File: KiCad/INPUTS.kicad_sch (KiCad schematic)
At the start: 8 parts

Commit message: Actualizació Footprints
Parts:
- R_BTNDOWN1, R_BTNUP1, R_LIMIT1, R_MCLR1: footprint (none) -> Resistor_SMD:R_0805_2012Metric
- SW_UP1, SW_UP2, SW_UP3, SW_UP4: footprint (none) -> Button_Switch_SMD:SW_SPST_TL3342
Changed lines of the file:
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@@
 			)
 		)
-		(property "Footprint" ""
+		(property "Footprint" "Resistor_SMD:R_0805_2012Metric"
 			(at 139.7 74.168 90)
 			(effects
@@
 			)
 		)
-		(property "Footprint" ""
+		(property "Footprint" "Resistor_SMD:R_0805_2012Metric"
 			(at 139.7 95.758 90)
 			(effects
@@
 			)
 		)
-		(property "Footprint" ""
+		(property "Footprint" "Button_Switch_SMD:SW_SPST_TL3342"
 			(at 152.4 67.31 0)
 			(effects
@@
 			)
 		)
-		(property "Footprint" ""
+		(property "Footprint" "Resistor_SMD:R_0805_2012Metric"
 			(at 139.7 117.348 90)
 			(effects
@@
 			)
 		)
-		(property "Footprint" ""
+		(property "Footprint" "Resistor_SMD:R_0805_2012Metric"
 			(at 139.7 51.308 90)
 			(effects
@@
 			)
 		)
-		(property "Footprint" ""
+		(property "Footprint" "Button_Switch_SMD:SW_SPST_TL3342"
 			(at 152.4 88.9 0)
 			(effects
@@
 			)
 		)
-		(property "Footprint" ""
+		(property "Footprint" "Button_Switch_SMD:SW_SPST_TL3342"
 			(at 152.4 110.49 0)
 			(effects
@@
 			)
 		)
-		(property "Footprint" ""
+		(property "Footprint" "Button_Switch_SMD:SW_SPST_TL3342"
 			(at 152.4 44.45 0)
 			(effects

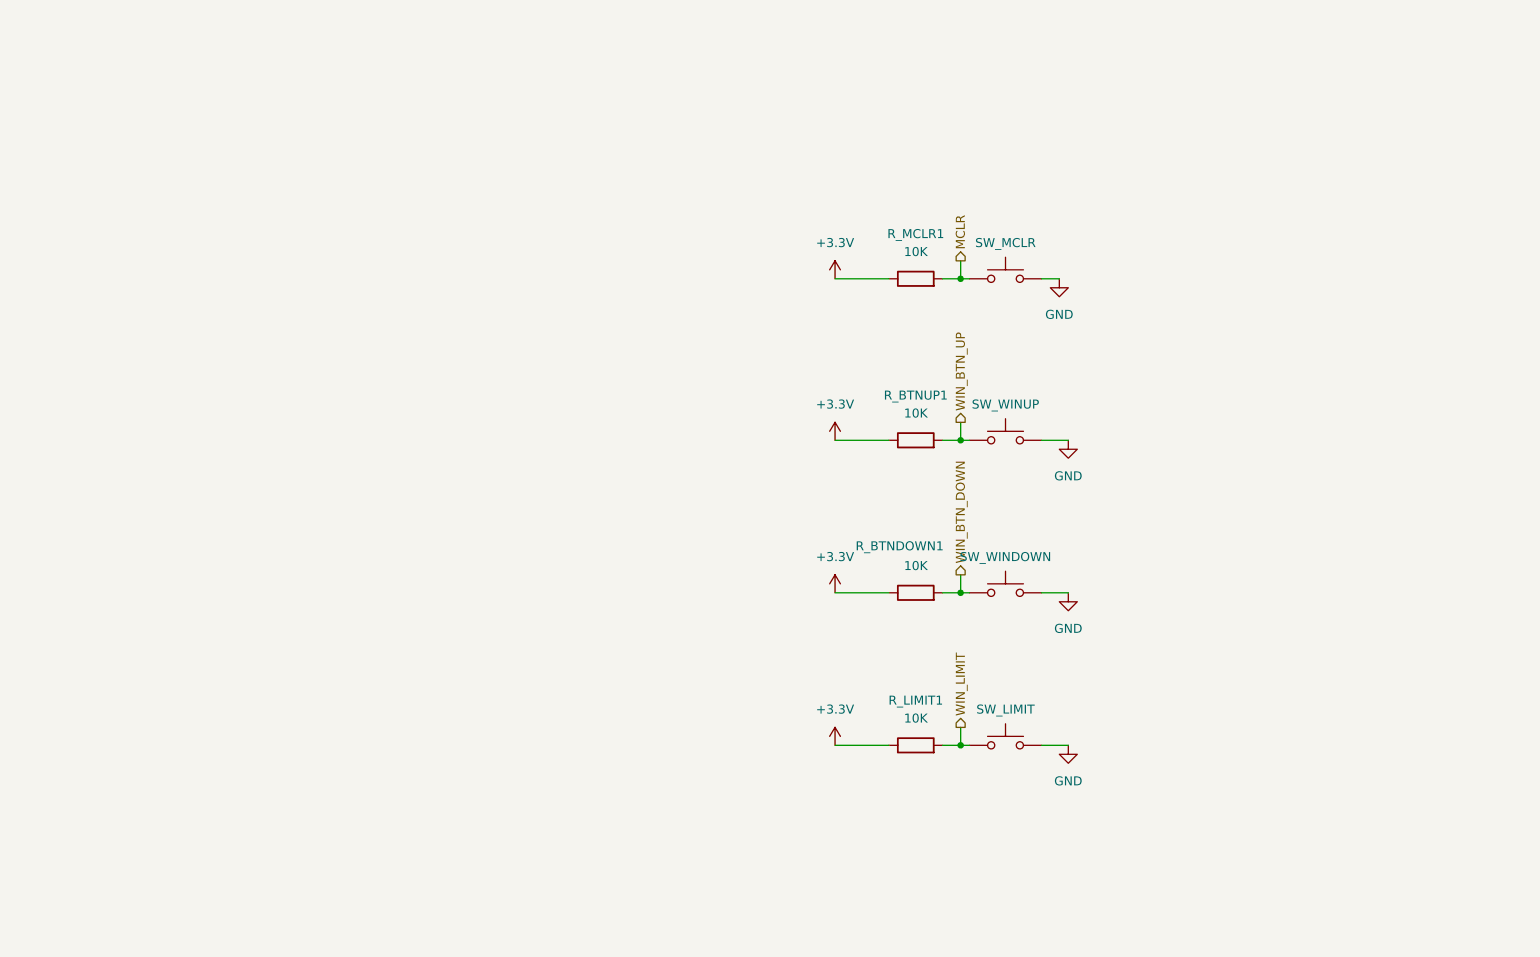
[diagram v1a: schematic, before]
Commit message: Versió final Esquematic
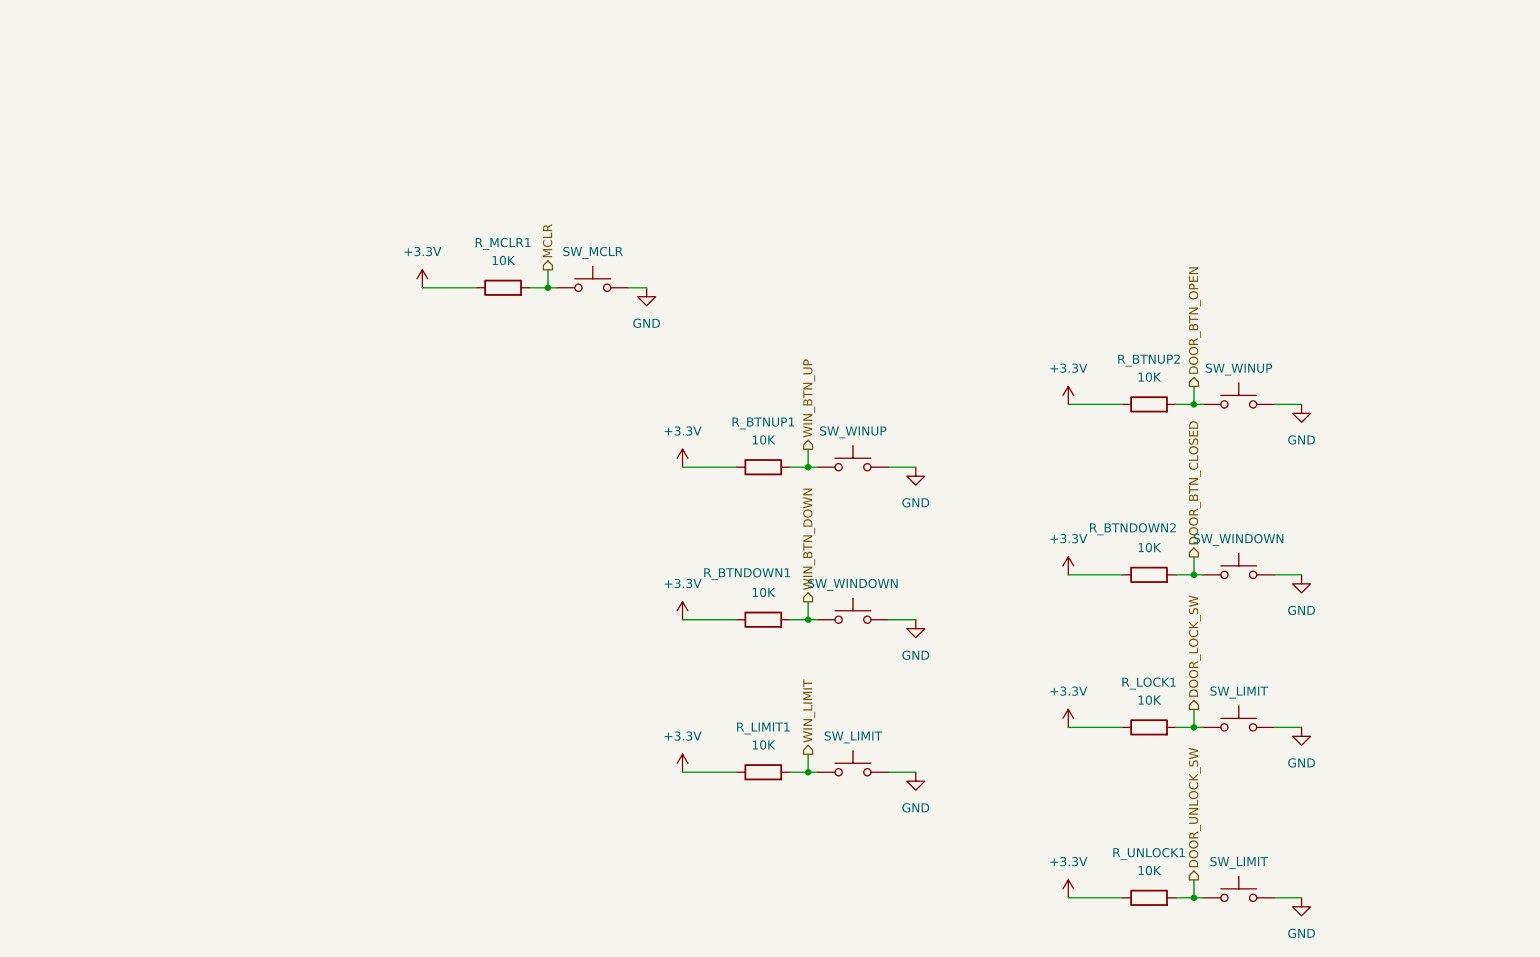
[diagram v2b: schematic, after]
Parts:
- added R_BTNDOWN2, R_BTNUP2, R_LOCK1, R_UNLOCK1: 10K, Resistor_SMD:R_0805_2012Metric, symbol Device:R
- added SW_UP5: SW_WINUP, Button_Switch_SMD:SW_SPST_TL3342, symbol Switch:SW_Push
- added SW_UP6: SW_WINDOWN, Button_Switch_SMD:SW_SPST_TL3342, symbol Switch:SW_Push
- added SW_UP7, SW_UP8: SW_LIMIT, Button_Switch_SMD:SW_SPST_TL3342, symbol Switch:SW_Push
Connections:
- net +3.3V: now also R_BTNDOWN2.1, R_BTNUP2.1, R_LOCK1.1, R_UNLOCK1.1
- net GND: now also SW_UP5.2, SW_UP6.2, SW_UP7.2, SW_UP8.2
- new net DOOR_BTN_CLOSED: R_BTNDOWN2.2, SW_UP6.1
- new net DOOR_BTN_OPEN: R_BTNUP2.2, SW_UP5.1
- new net DOOR_LOCK_SW: R_LOCK1.2, SW_UP7.1
- new net DOOR_UNLOCK_SW: R_UNLOCK1.2, SW_UP8.1
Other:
- moved on the sheet: R_BTNDOWN1, R_BTNUP1, R_LIMIT1, R_MCLR1

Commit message: Versió final de l'esquematic
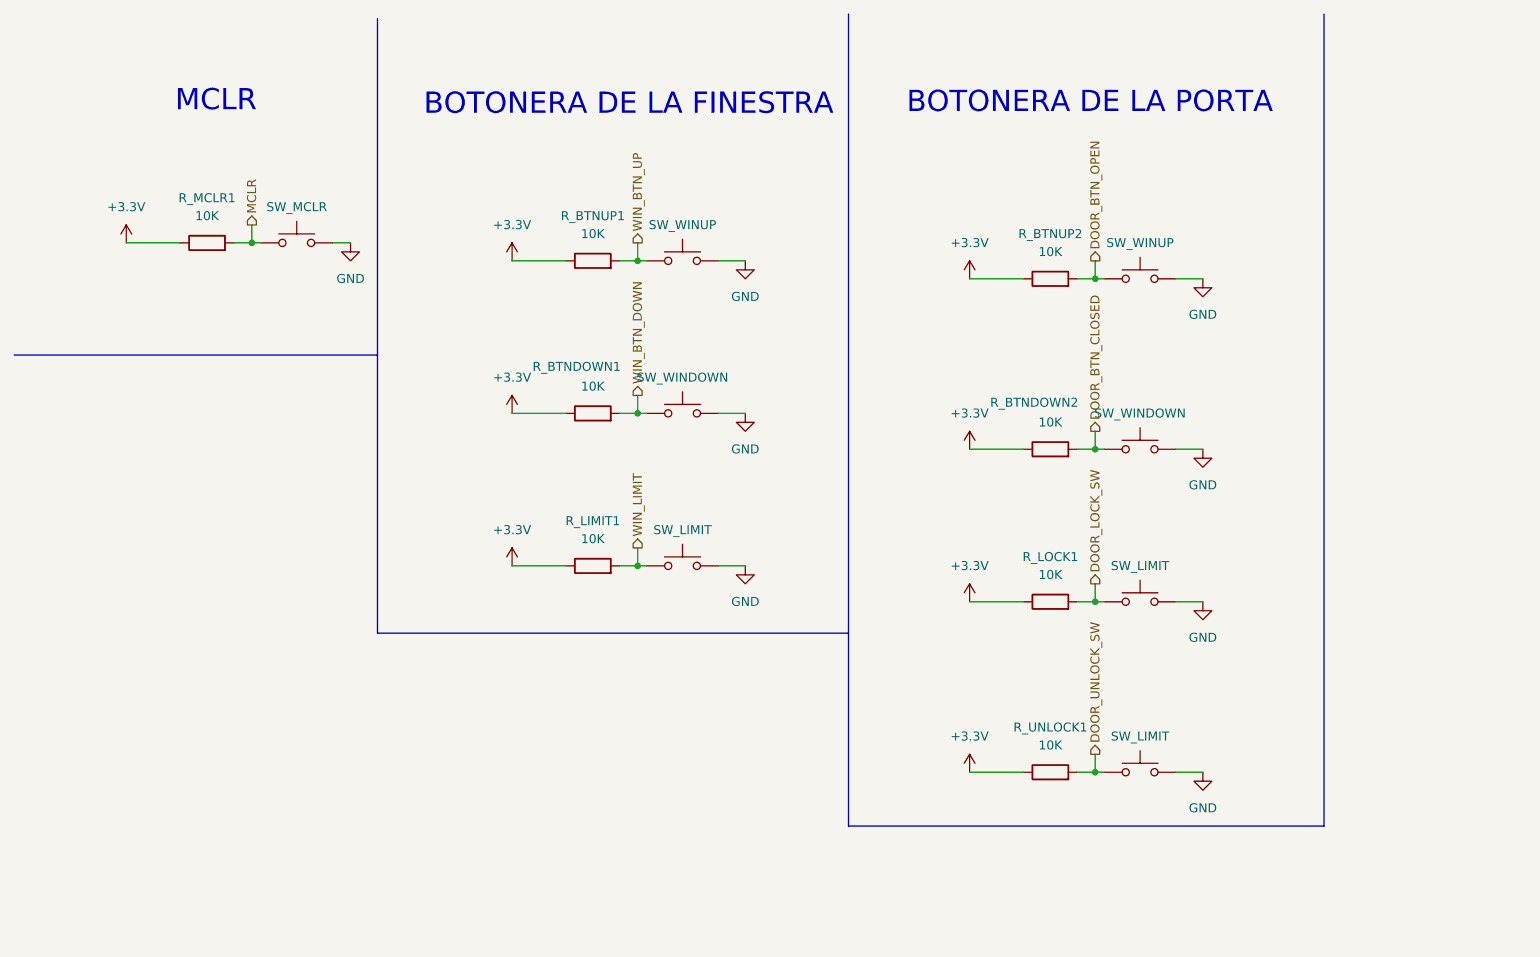
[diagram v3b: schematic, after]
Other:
- note added: "BOTONERA DE LA FINESTRA"
- note added: "BOTONERA DE LA PORTA"
- note added: "MCLR"
- moved on the sheet: R_BTNDOWN1, R_BTNDOWN2, R_BTNUP1, R_BTNUP2, R_LIMIT1, R_LOCK1, R_MCLR1, R_UNLOCK1

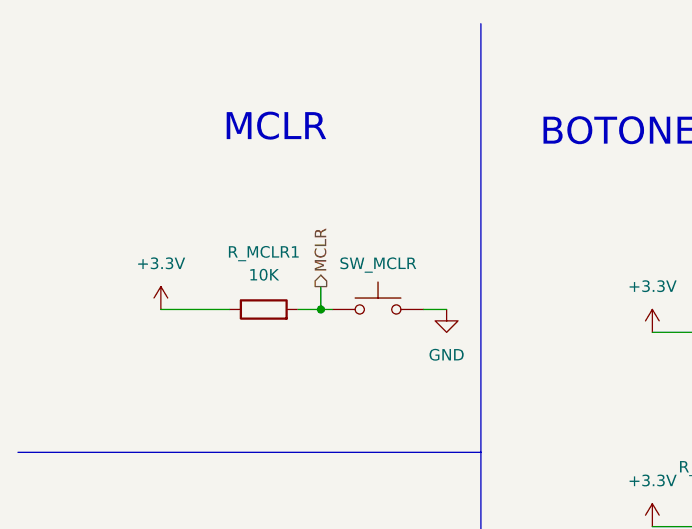
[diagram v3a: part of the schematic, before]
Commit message: 1ra versióPCB
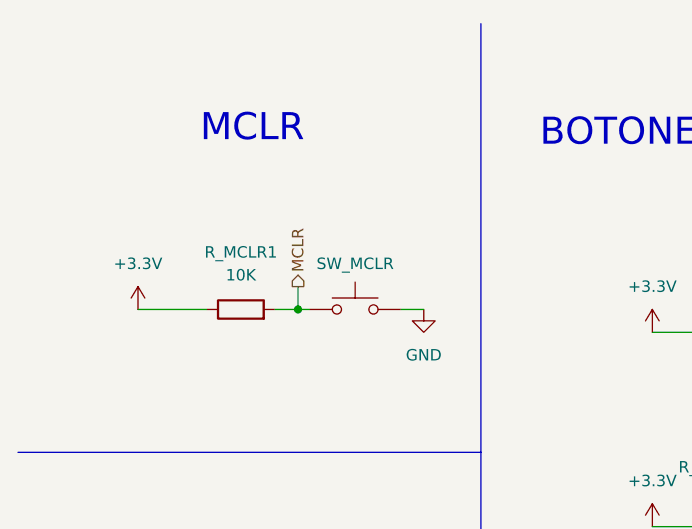
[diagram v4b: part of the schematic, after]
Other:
- moved on the sheet: R_MCLR1
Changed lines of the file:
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@@
 	(text "MCLR"
 		(exclude_from_sim no)
-		(at 40.64 24.384 0)
+		(at 38.1 24.384 0)
 		(effects
 			(font
@@
 	)
 	(junction
-		(at 45.72 44.45)
+		(at 43.18 44.45)
 		(diameter 0)
 		(color 0 0 0 0)
@@
 	(wire
 		(pts
-			(xy 57.15 44.45) (xy 59.69 44.45)
-		)
-		(stroke
-			(width 0)
-			(type default)
-		)
-	)
-	(wire
-		(pts
-			(xy 43.18 44.45) (xy 45.72 44.45)
+			(xy 54.61 44.45) (xy 57.15 44.45)
+		)
+		(stroke
+			(width 0)
+			(type default)
+		)
+	)
+	(wire
+		(pts
+			(xy 40.64 44.45) (xy 43.18 44.45)
 		)
 		(stroke
@@
 	(wire
 		(pts
-			(xy 45.72 41.91) (xy 45.72 44.45)
+			(xy 43.18 41.91) (xy 43.18 44.45)
 		)
 		(stroke
@@
 	(wire
 		(pts
-			(xy 27.94 44.45) (xy 35.56 44.45)
+			(xy 25.4 44.45) (xy 33.02 44.45)
 		)
 		(stroke
@@
 	(wire
 		(pts
-			(xy 45.72 44.45) (xy 46.99 44.45)
+			(xy 43.18 44.45) (xy 44.45 44.45)
 		)
 		(stroke
@@
 	(hierarchical_label "MCLR"
 		(shape output)
-		(at 45.72 41.91 90)
+		(at 43.18 41.91 90)
 		(effects
 			(font
@@
 	(symbol
 		(lib_id "power:+3.3V")
-		(at 27.94 44.45 0)
+		(at 25.4 44.45 0)
 		(unit 1)
 		(exclude_from_sim no)
@@
 		(fields_autoplaced yes)
 		(property "Reference" "#PWR022"
-			(at 27.94 48.26 0)
+			(at 25.4 48.26 0)
 			(effects
 				(font
@@
 		)
 		(property "Value" "+3.3V"
-			(at 27.94 39.37 0)
+			(at 25.4 39.37 0)
 			(effects
 				(font
@@
 		)
 		(property "Footprint" ""
-			(at 27.94 44.45 0)
+			(at 25.4 44.45 0)
 			(effects
 				(font
@@
 		)
 		(property "Datasheet" ""
-			(at 27.94 44.45 0)
+			(at 25.4 44.45 0)
 			(effects
 				(font
@@
 		)
 		(property "Description" "Power symbol creates a global label with name \"+3.3V\""
-			(at 27.94 44.45 0)
+			(at 25.4 44.45 0)
 			(effects
 				(font
@@
 	(symbol
 		(lib_id "Device:R")
-		(at 39.37 44.45 90)
+		(at 36.83 44.45 90)
 		(unit 1)
 		(exclude_from_sim no)
@@
 		(fields_autoplaced yes)
 		(property "Reference" "R_MCLR1"
-			(at 39.37 38.1 90)
+			(at 36.83 38.1 90)
 			(effects
 				(font
@@
 		)
 		(property "Value" "10K"
-			(at 39.37 40.64 90)
+			(at 36.83 40.64 90)
 			(effects
 				(font
@@
 		)
 		(property "Footprint" "Resistor_SMD:R_0805_2012Metric"
-			(at 39.37 46.228 90)
+			(at 36.83 46.228 90)
 			(effects
 				(font
@@
 		)
 		(property "Datasheet" "~"
-			(at 39.37 44.45 0)
+			(at 36.83 44.45 0)
 			(effects
 				(font
@@
 		)
 		(property "Description" "Resistor"
-			(at 39.37 44.45 0)
+			(at 36.83 44.45 0)
 			(effects
 				(font
@@
 	(symbol
 		(lib_id "Switch:SW_Push")
-		(at 52.07 44.45 0)
+		(at 49.53 44.45 0)
 		(unit 1)
 		(exclude_from_sim no)
@@
 		(fields_autoplaced yes)
 		(property "Reference" "SW_UP1"
-			(at 52.07 36.83 0)
+			(at 49.53 36.83 0)
 			(effects
 				(font
@@
 		)
 		(property "Value" "SW_MCLR"
-			(at 52.07 39.37 0)
+			(at 49.53 39.37 0)
 			(effects
 				(font
@@
 		)
 		(property "Footprint" "Button_Switch_SMD:SW_SPST_TL3342"
-			(at 52.07 39.37 0)
+			(at 49.53 39.37 0)
 			(effects
 				(font
@@
 		)
 		(property "Datasheet" "~"
-			(at 52.07 39.37 0)
+			(at 49.53 39.37 0)
 			(effects
 				(font
@@
 		)
 		(property "Description" "Push button switch, generic, two pins"
-			(at 52.07 44.45 0)
+			(at 49.53 44.45 0)
 			(effects
 				(font
@@
 	(symbol
 		(lib_id "power:GND")
-		(at 59.69 44.45 0)
+		(at 57.15 44.45 0)
 		(unit 1)
 		(exclude_from_sim no)
@@
 		(fields_autoplaced yes)
 		(property "Reference" "#PWR023"
-			(at 59.69 50.8 0)
+			(at 57.15 50.8 0)
 			(effects
 				(font
@@
 		)
 		(property "Value" "GND"
-			(at 59.69 49.53 0)
+			(at 57.15 49.53 0)
 			(effects
 				(font
@@
 		)
 		(property "Footprint" ""
-			(at 59.69 44.45 0)
+			(at 57.15 44.45 0)
 			(effects
 				(font
@@
 		)
 		(property "Datasheet" ""
-			(at 59.69 44.45 0)
+			(at 57.15 44.45 0)
 			(effects
 				(font
@@
 		)
 		(property "Description" "Power symbol creates a global label with name \"GND\" , ground"
-			(at 59.69 44.45 0)
-			(effects
-				(font
+			(at 57.15 44.45 0)
+			(effects
+				(font
